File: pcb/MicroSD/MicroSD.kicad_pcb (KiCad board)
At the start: 2 copper layers, 14 parts, among them J1 Micro_SD_Card, J2 Conn_01x06_MountingPin, U1 74LVC125A, U2 AMS1117

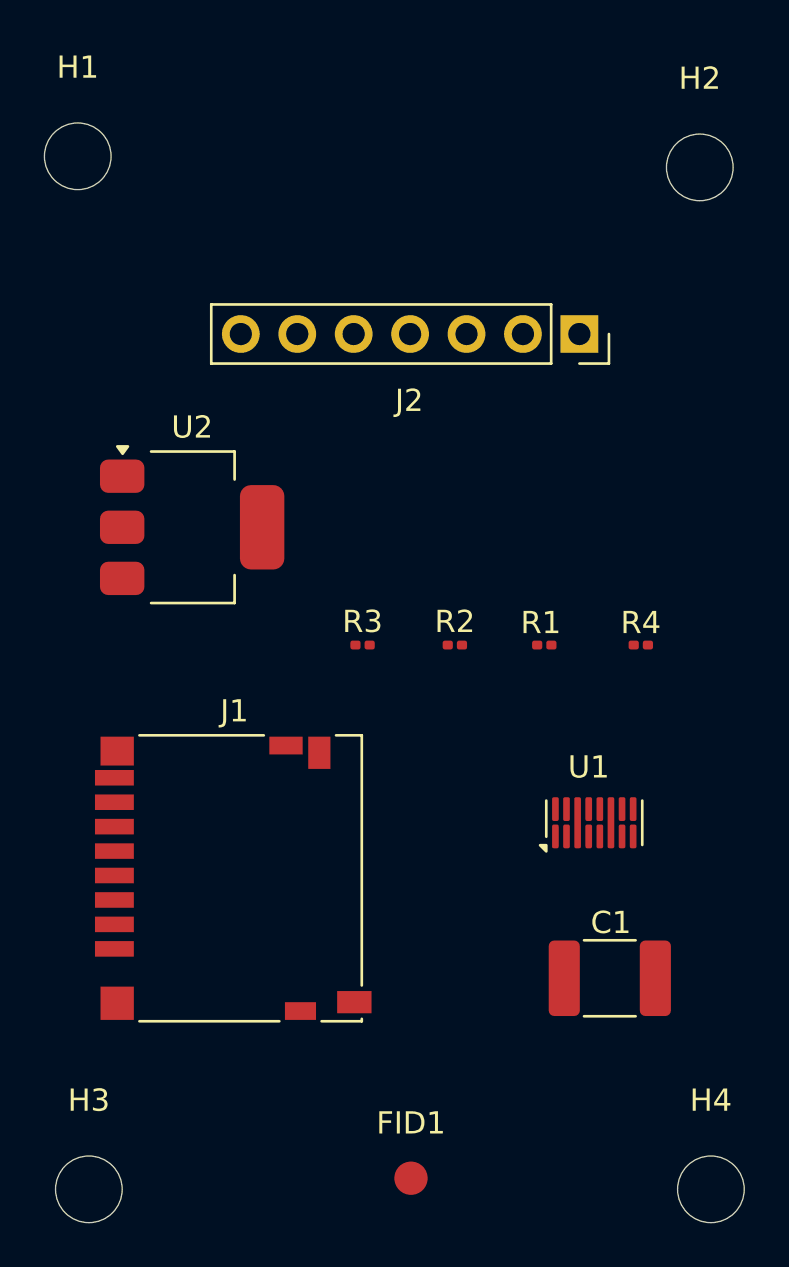
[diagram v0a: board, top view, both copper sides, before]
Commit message: se actualiza PCB y esquemas
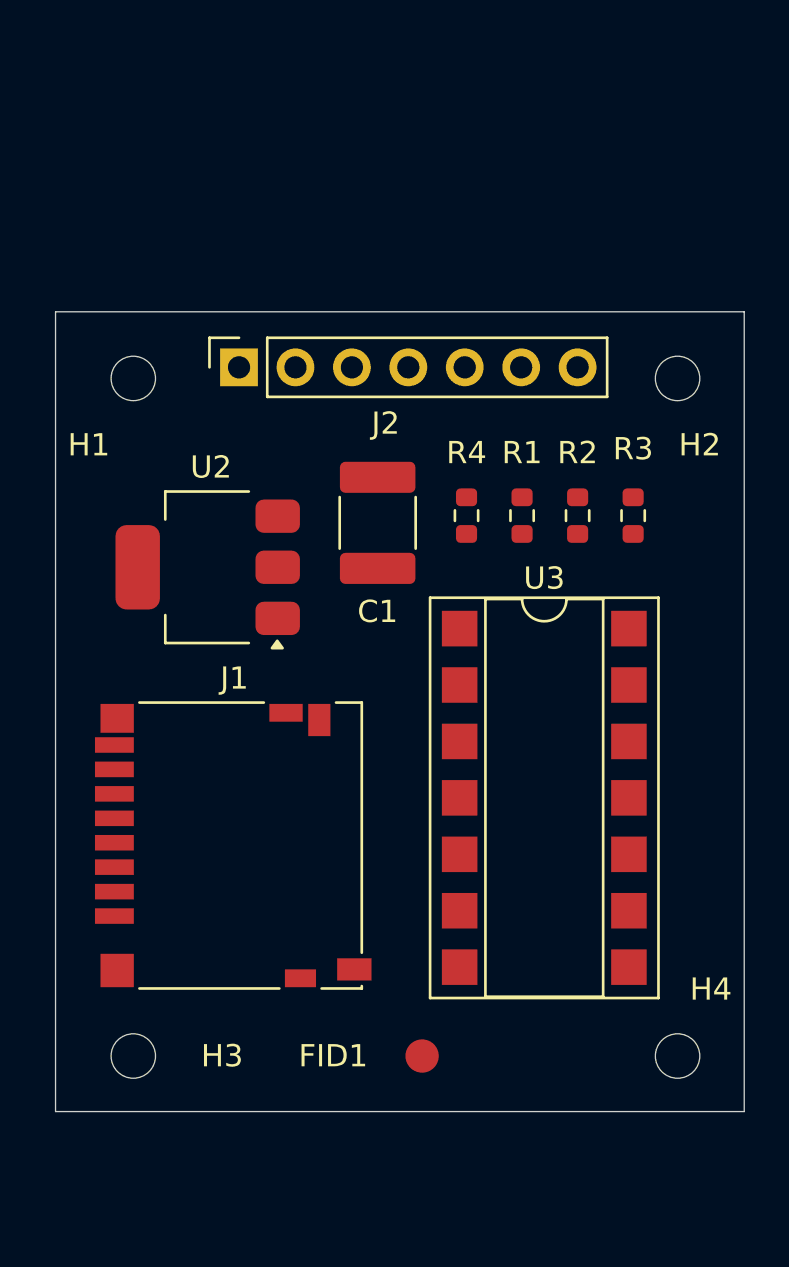
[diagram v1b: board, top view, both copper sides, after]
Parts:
- removed U1: 74LVC125A, Package_TO_SOT_SMD:SOT-1334-1
- added U3: 74LVC125, Package_DIP:DIP-14_W7.62mm_SMDSocket_SmallPads, F.Cu at (136.0, 97.9)
- H1, H2, H3, H4: footprint MountingHole:MountingHole_3mm -> MountingHole:MountingHole_2mm
- R1, R2, R3, R4: footprint Resistor_SMD:R_0201_0603Metric -> Resistor_SMD:R_0603_1608Metric
- moved C1 23.0 mm to (128.5, 85.5), turned to 90 degrees
- moved J2 15.4 mm to (122.3, 78.5), turned to 90 degrees
- moved R3 13.5 mm to (140.0, 85.2), turned to -90 degrees
- moved H1 10.3 mm to (117.5, 79.0)
- moved R4 9.77 mm to (132.5, 85.2), turned to 90 degrees
- moved H2 9.55 mm to (142.0, 79.0)
- moved R2 8.03 mm to (137.5, 85.2), turned to -90 degrees
- moved H3 6.32 mm to (117.5, 109.5)
- moved H4 6.18 mm to (142.0, 109.5)
- moved R1 5.91 mm to (135.0, 85.2), turned to -90 degrees
- moved FID1 5.52 mm to (130.5, 109.5)
- moved U2 1.93 mm to (120.8, 87.5), turned to 180 degrees
- moved J1 1.47 mm to (122.0, 100.0)
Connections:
- net /VDD renamed VDD
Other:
- board outline added: 31 x 36 mm

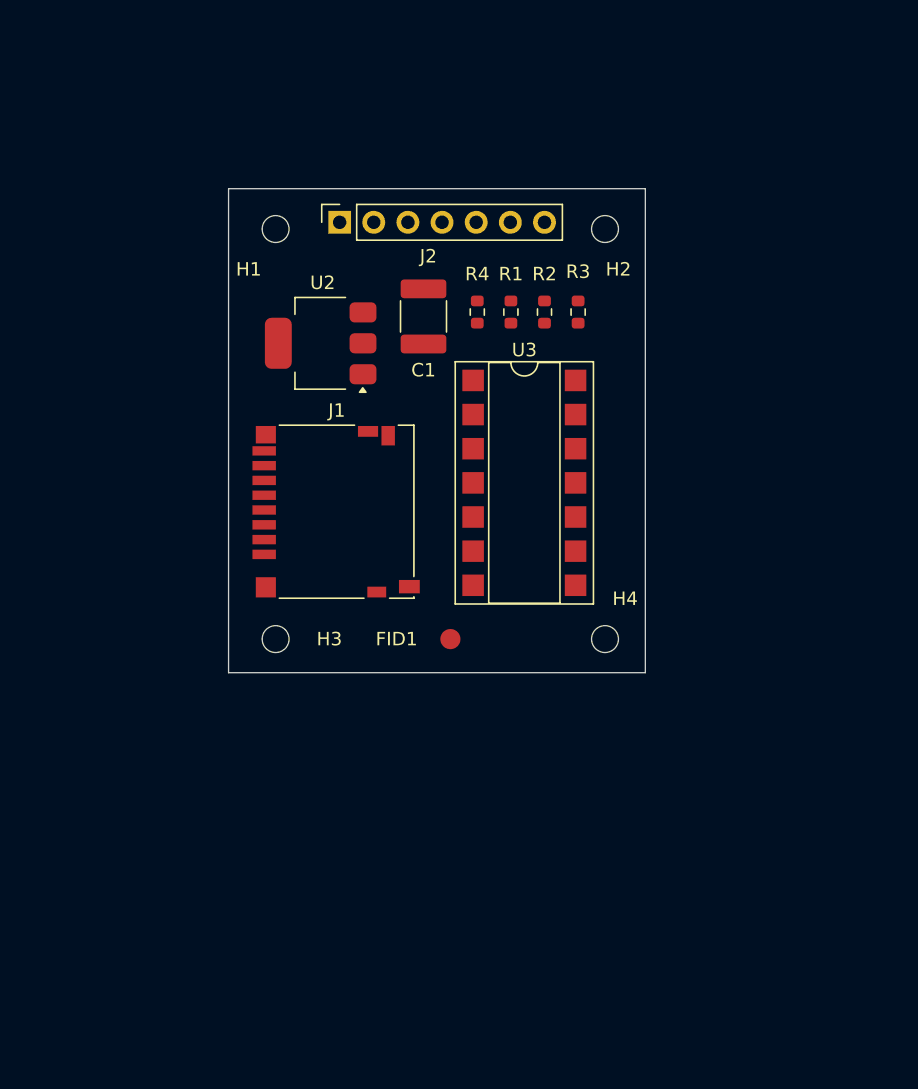
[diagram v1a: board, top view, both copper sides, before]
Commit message: se actualiza PCB y esquemas 2
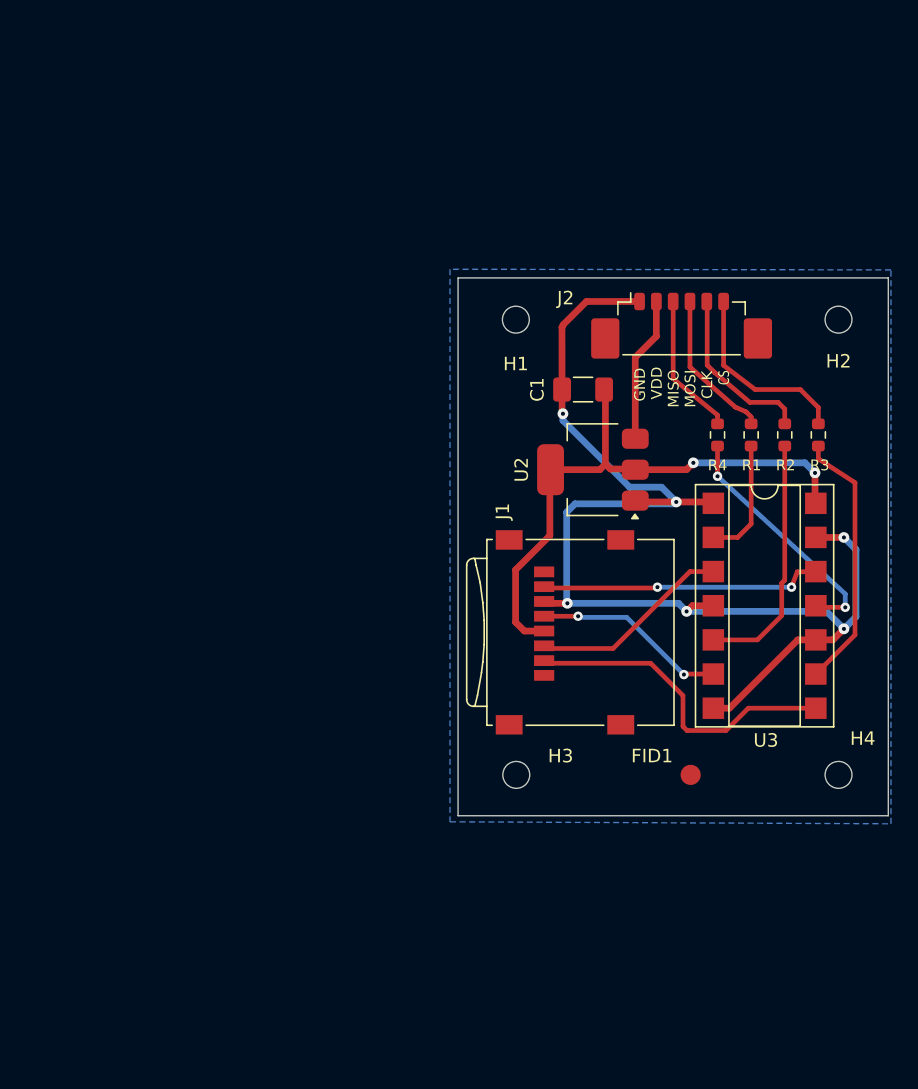
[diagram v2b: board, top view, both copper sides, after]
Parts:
- C1: footprint Capacitor_SMD:C_1812_4532Metric -> Capacitor_SMD:C_1206_3216Metric_Pad1.33x1.80mm_HandSolder
- J1: footprint Connector_Card:microSD_HC_Hirose_DM3D-SF -> Connector_Card:microSD_HC_Wuerth_693072010801
- J2: footprint Connector_PinSocket_2.54mm:PinSocket_1x07_P2.54mm_Vertical -> Connector_Molex:Molex_PicoBlade_53398-0671_1x06-1MP_P1.25mm_Vertical
- moved J2 26.4 mm to (147.7, 85.6), turned to 0 degrees
- moved U2 22.3 mm to (141.1, 96.9)
- moved H3 20.6 mm to (135.4, 119.6)
- moved FID1 20.5 mm to (148.4, 119.6)
- moved H4 20.1 mm to (159.4, 119.6)
- moved R1 20.1 mm to (152.9, 94.3)
- moved R2 20.1 mm to (155.4, 94.3)
- moved R3 20.1 mm to (157.9, 94.3)
- moved R4 20.1 mm to (150.4, 94.3)
- moved U3 20.1 mm to (153.9, 107.0)
- moved J1 19.2 mm to (139.0, 109.0), turned to 90 degrees
- moved H1 19.1 mm to (135.4, 85.7)
- moved H2 18.6 mm to (159.4, 85.7)
- moved C1 13.1 mm to (140.4, 90.9), turned to 180 degrees
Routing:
- net GND: track 0.00 -> 92.9 mm, vias 0 -> 6
- net VDD: track 0.00 -> 43.7 mm, vias 0 -> 2
- net /DAT3/CD: track 0.00 -> 24.8 mm
- net Net-(J1-DAT0): track 0.00 -> 21.6 mm, vias 0 -> 2
- net Net-(R3-Pad2): track 0.00 -> 19.6 mm
- net Net-(R2-Pad2): track 0.00 -> 18.5 mm
- net Net-(R4-Pad1): track 0.00 -> 18.4 mm, vias 0 -> 2
- net Net-(J1-CMD): track 0.00 -> 15.5 mm
- net Net-(J1-CLK): track 0.00 -> 14.4 mm, vias 0 -> 2
- net Net-(J2-Pin_6): track 0.00 -> 14.2 mm
- net Net-(J2-Pin_5): track 0.00 -> 12.9 mm
- net Net-(J2-Pin_4): track 0.00 -> 11.3 mm
- net Net-(J2-Pin_2): track 0.00 -> 11.0 mm
- net /PIN3: track 0.00 -> 10.7 mm
- net Net-(R1-Pad2): track 0.00 -> 9.02 mm
- added copper zone on B.Cu, net GND
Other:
- board size 31 x 36 mm -> 32 x 40 mm
- board text added: "0,0000 mm / 0,0000 mm"
- board text added: "0,3000 mm"
- board text added: "1,6000 mm"
- board text added: "2"
- board text added: "30,0000 mm x 40,0000 mm"
- board text added: "Bordes de la placa revestidos:"
- board text added: "CARACTERÍSTICAS DE LA PLACA"
- board text added: "CLK"
- board text added: "CS"
- board text added: "Conectores laterales de tarjeta:"
- board text added: "Control de impedancia:"
- board text added: "Dimensiones generales de la placa:"
- board text added: "Diámetro mínimo de orificio:"
- board text added: "GND"
- board text added: "Grosor de la placa:"
- board text added: "MISO"
- board text added: "MOSI"
- board text added: "Micro SD Card Adapter v0 2024-10-08"
- board text added: "No"
- board text added: "None"
- board text added: "Número de capas de cobre:"
- board text added: "Pads almena:"
- board text added: "Pista/espaciado mínimo:"
- board text added: "Terminación de cobre:"
- board text added: "VDD"

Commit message: se actualiza resultados
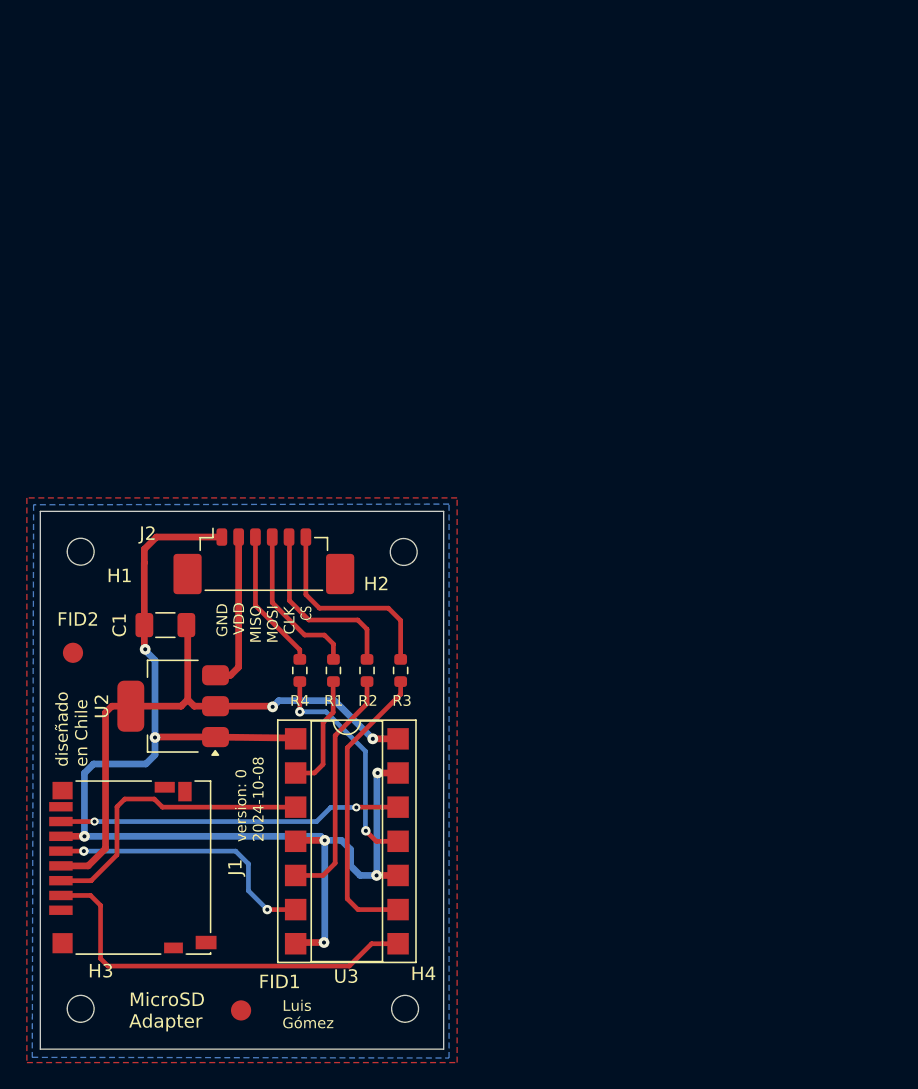
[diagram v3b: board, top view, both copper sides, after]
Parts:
- added FID2: Fiducial, Fiducial:Fiducial_1.5mm_Mask3mm, F.Cu at (102.4, 110.5)
- J1: footprint Connector_Card:microSD_HC_Wuerth_693072010801 -> Connector_Card:microSD_HC_Hirose_DM3D-SF
- moved FID1 37.8 mm to (114.9, 137.1)
- moved H3 36.8 mm to (103.0, 137.0)
- moved H1 36.7 mm to (103.0, 103.0)
- moved H2 36.7 mm to (127.0, 103.0)
- moved H4 36.6 mm to (127.1, 137.0)
- moved J1 36.6 mm to (106.9, 126.5), turned to -90 degrees
- moved U2 35.8 mm to (109.9, 114.5)
- moved U3 35.7 mm to (122.8, 124.5)
- moved C1 35.7 mm to (109.3, 108.5)
- moved R1 35.7 mm to (121.8, 111.8)
- moved R2 35.7 mm to (124.3, 111.8)
- moved R3 35.7 mm to (126.8, 111.8)
- moved R4 35.7 mm to (119.3, 111.8)
- moved J2 35.7 mm to (116.6, 103.2)
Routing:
- net Net-(J1-CMD): track 15.5 -> 22.3 mm
- net Net-(J1-CLK): track 14.4 -> 20.4 mm
- net /DAT3/CD: track 24.8 -> 30.3 mm
- net Net-(J1-DAT0): track 21.6 -> 25.5 mm
- net GND: track 92.9 -> 90.5 mm, vias 6 -> 7
- net Net-(R3-Pad2): track 19.6 -> 21.9 mm
- net Net-(R4-Pad1): track 18.4 -> 17.0 mm
- net Net-(J2-Pin_6): track 14.2 -> 15.0 mm
- net Net-(R2-Pad2): track 18.5 -> 17.8 mm
- net Net-(J2-Pin_5): track 12.9 -> 13.6 mm
- net Net-(J2-Pin_2): track 11.0 -> 11.6 mm
- net Net-(J2-Pin_4): track 11.3 -> 11.8 mm
- net VDD: track 43.7 -> 43.2 mm
- added copper zone on F.Cu, net GND
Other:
- board size 32 x 40 mm -> 30 x 40 mm
- board text added: "0,2500 mm / 0,2000 mm"
- board text added: "Luis Gómez"
- board text added: "Línea de seguridad"
- board text added: "MicroSD Adapter"
- board text added: "diseñado en Chile"
- board text added: "version: 0 2024-10-08"
- board text removed: "0,0000 mm / 0,0000 mm"
- board text removed: "Micro SD Card Adapter v0 2024-10-08"
